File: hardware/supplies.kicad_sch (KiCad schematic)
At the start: 20 parts, among them J11 Conn_01x02, J12 Conn_01x02, U8 AP62250WU

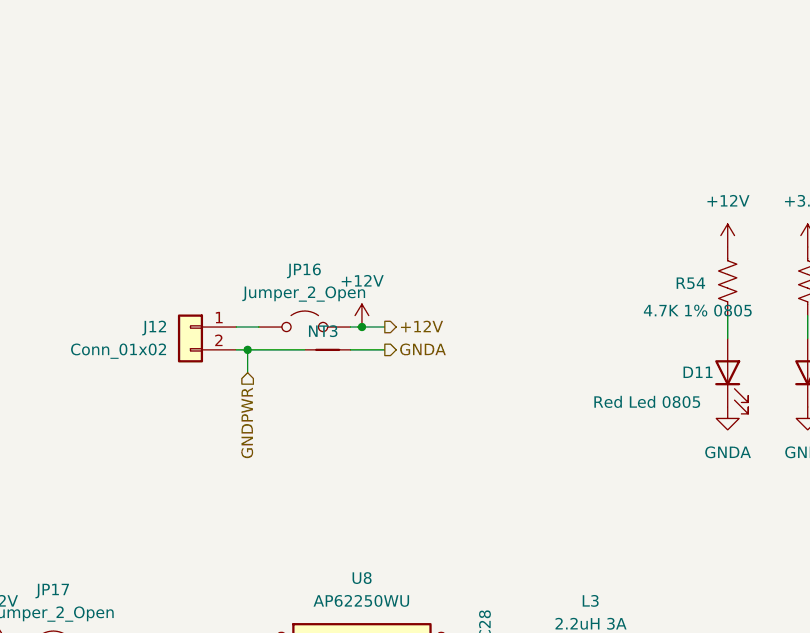
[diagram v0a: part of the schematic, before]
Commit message: HW: PCB Done
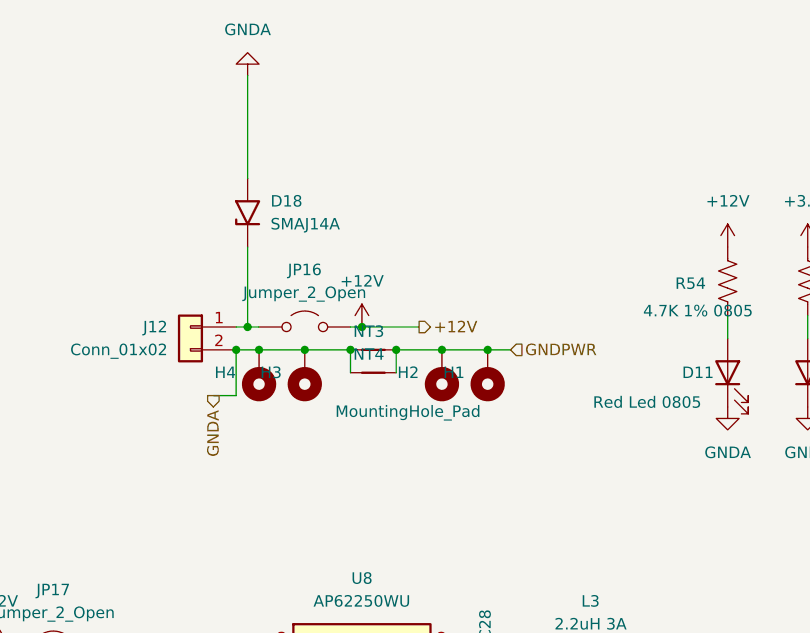
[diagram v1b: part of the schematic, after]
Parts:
- added D18: SMAJ14A, Diode_SMD:D_SMA, symbol Diode:SMAJ14A
- added H1, H2, H3, H4: MountingHole_Pad, MountingHole:MountingHole_3.2mm_M3_Pad, symbol Mechanical:MountingHole_Pad
- added NT4: NetTie_2, NetTie:NetTie-2_SMD_Pad2.0mm, symbol Device:NetTie_2
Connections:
- net GNDA: now also J12.2 (Pin_2), NT3.1, D18.2 (A2), H3.1, H4.1, NT4.1; no longer NT3.2
- net GNDPWR: now also NT3.2, H1.1, H2.1, NT4.2; no longer J12.2 (Pin_2), NT3.1
- net at J12.1 (Pin_1), JP16.2 (B): now also D18.1 (A1)
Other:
- moved on the sheet: NT3
